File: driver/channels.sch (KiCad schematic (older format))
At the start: 2 parts, among them J201 A_1_32, J202 K_1_32

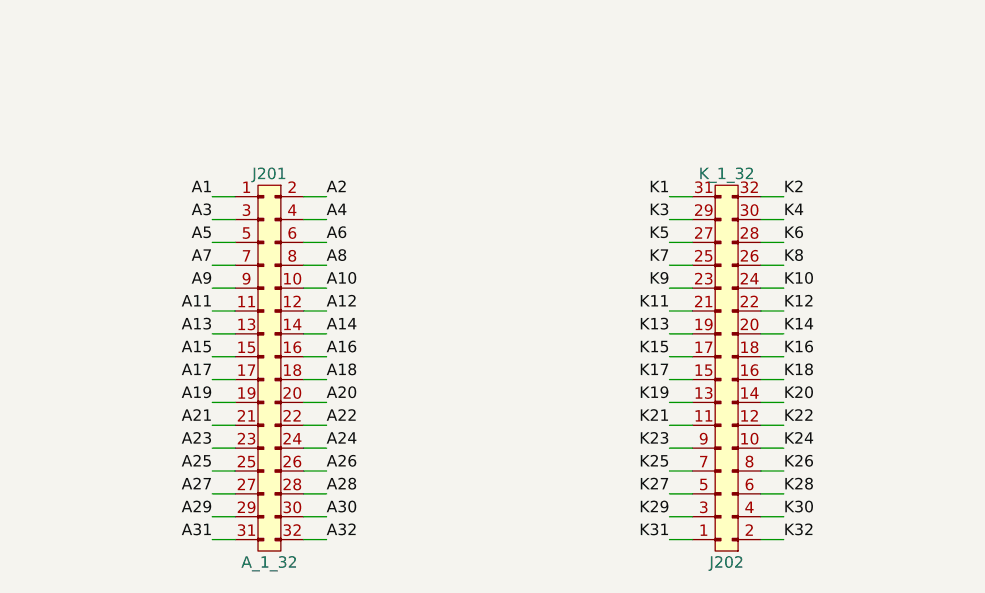
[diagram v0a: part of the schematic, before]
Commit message: WIP routing driver
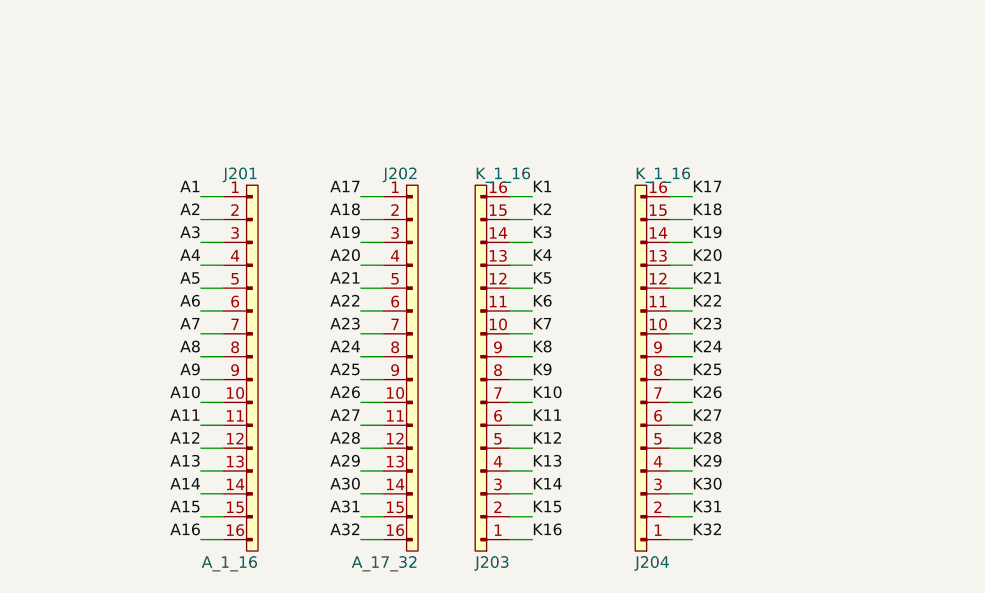
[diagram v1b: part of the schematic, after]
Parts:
- removed J201: A_1_32, agg:DIL-254P-32, symbol agg-kicad:CONN_02x16
- removed J202: K_1_32, agg:DIL-254P-32, symbol agg-kicad:CONN_02x16
- added J201: A_1_16, agg:IPL1-116-02-L-SH, symbol agg-kicad:CONN_01x16
- added J202: A_17_32, agg:IPL1-116-02-L-SH, symbol agg-kicad:CONN_01x16
- added J203, J204: K_1_16, agg:IPL1-116-02-L-SH, symbol agg-kicad:CONN_01x16
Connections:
- net A1: now also J201.1
- net A10: now also J201.10
- net A11: now also J201.11
- net A12: now also J201.12
- net A13: now also J201.13
- net A14: now also J201.14
- net A15: now also J201.15
- net A16: now also J201.16
- net A17: now also J202.1
- net A18: now also J202.2
- net A19: now also J202.3
- net A2: now also J201.2
- net A20: now also J202.4
- net A21: now also J202.5
- net A22: now also J202.6
- net A23: now also J202.7
- net A24: now also J202.8
- net A25: now also J202.9
- net A26: now also J202.10
- net A27: now also J202.11
- net A28: now also J202.12
- net A29: now also J202.13
- net A3: now also J201.3
- net A30: now also J202.14
- net A31: now also J202.15
- net A32: now also J202.16
- net A4: now also J201.4
- net A5: now also J201.5
- net A6: now also J201.6
- net A7: now also J201.7
- net A8: now also J201.8
- net A9: now also J201.9
- net K1: now also J203.16
- net K10: now also J203.7
- net K11: now also J203.6
- net K12: now also J203.5
- net K13: now also J203.4
- net K14: now also J203.3
- net K15: now also J203.2
- net K16: now also J203.1
- net K17: now also J204.16
- net K18: now also J204.15
- net K19: now also J204.14
- net K2: now also J203.15
- net K20: now also J204.13
- net K21: now also J204.12
- net K22: now also J204.11
- net K23: now also J204.10
- net K24: now also J204.9
- net K25: now also J204.8
- net K26: now also J204.7
- net K27: now also J204.6
- net K28: now also J204.5
- net K29: now also J204.4
- net K3: now also J203.14
- net K30: now also J204.3
- net K31: now also J204.2
- net K32: now also J204.1
- net K4: now also J203.13
- net K5: now also J203.12
- net K6: now also J203.11
- net K7: now also J203.10
- net K8: now also J203.9
- net K9: now also J203.8
